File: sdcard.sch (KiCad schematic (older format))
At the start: 8 parts, among them J10 Micro_SD_Card

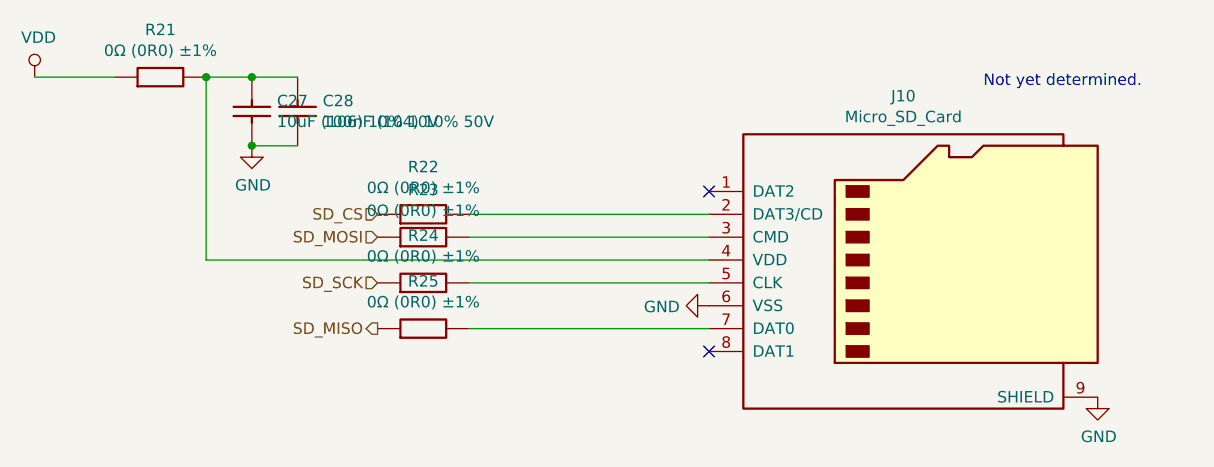
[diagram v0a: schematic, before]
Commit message: 20191114
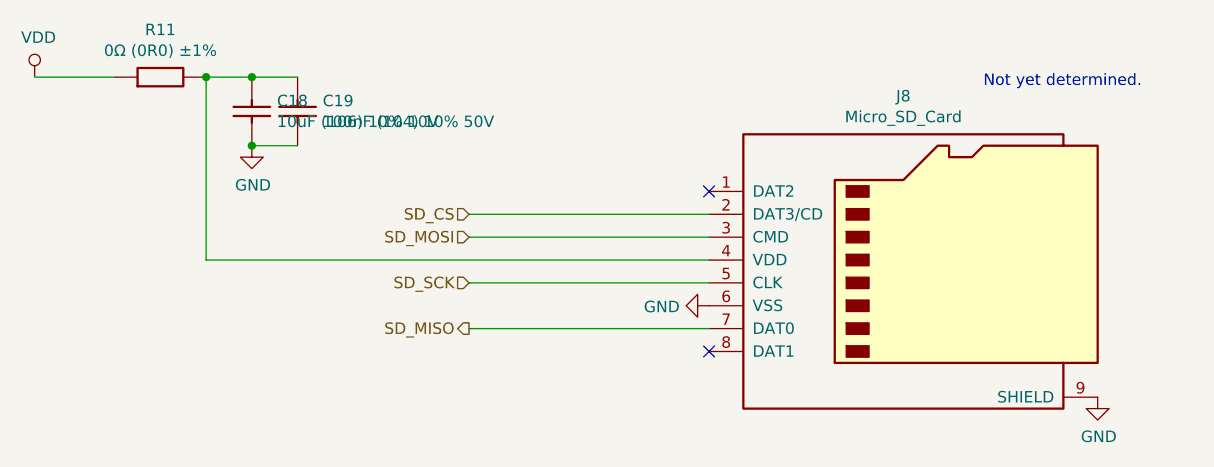
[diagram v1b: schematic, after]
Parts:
- removed R22, R23, R24, R25: 0603_0Ω__0R0_1%, lc_lib:0603_R, symbol lc_RES:0603_0Ω__0R0_1%
- J8: renamed from J10; footprint (none) -> Connector_Card:microSD_HC_Hirose_DM3D-SF
- renumbered C27 to C18, C28 to C19, R21 to R11
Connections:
- net SD_CS: now also J8.2 (DAT3/CD)
- net SD_MISO: now also J8.7 (DAT0)
- net SD_MOSI: now also J8.3 (CMD)
- net SD_SCK: now also J8.5 (CLK)
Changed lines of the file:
@@
 $Descr A4 11693 8268
 encoding utf-8
-Sheet 5 9
+Sheet 4 9
 Title ""
 Date ""
@@
 Comment4 ""
 $EndDescr
-Text HLabel 3550 3700 0    50   Output ~ 0
+Text HLabel 3950 3700 0    50   Output ~ 0
 SD_MISO
-Text HLabel 3550 3200 0    50   Input ~ 0
+Text HLabel 3950 3200 0    50   Input ~ 0
 SD_CS
-Text HLabel 3550 3300 0    50   Input ~ 0
+Text HLabel 3950 3300 0    50   Input ~ 0
 SD_MOSI
-Text HLabel 3550 3500 0    50   Input ~ 0
+Text HLabel 3950 3500 0    50   Input ~ 0
 SD_SCK
 $Comp
@@
 P 6700 4000
 AR Path="/5DF49590/5DCF2E63" Ref="#PWR?"  Part="1"
-AR Path="/5DCEE376/5DCF2E63" Ref="#PWR058"  Part="1"
-F 0 "#PWR058" H 6700 3750 50  0001 C CNN
+AR Path="/5DCEE376/5DCF2E63" Ref="#PWR038"  Part="1"
+F 0 "#PWR038" H 6700 3750 50  0001 C CNN
 F 1 "GND" H 6705 3827 50  0000 C CNN
 F 2 "" H 6700 4000 50  0001 C CNN
@@
 P 2600 2600
 AR Path="/5DF49590/5DCF2E76" Ref="R?"  Part="1"
-AR Path="/5DCEE376/5DCF2E76" Ref="R21"  Part="1"
-F 0 "R21" H 2600 2807 50  0000 C CNN
+AR Path="/5DCEE376/5DCF2E76" Ref="R11"  Part="1"
+F 0 "R11" H 2600 2807 50  0000 C CNN
 F 1 "0603_0Ω__0R0_1%" H 2450 2790 50  0001 L BNN
 F 2 "lc_lib:0603_R" H 2400 2360 50  0001 L BNN
@@
 P 5000 3600
 AR Path="/5DF49590/5DCF2EF5" Ref="#PWR?"  Part="1"
-AR Path="/5DCEE376/5DCF2EF5" Ref="#PWR057"  Part="1"
-F 0 "#PWR057" H 5000 3350 50  0001 C CNN
+AR Path="/5DCEE376/5DCF2EF5" Ref="#PWR037"  Part="1"
+F 0 "#PWR037" H 5000 3350 50  0001 C CNN
 F 1 "GND" V 5005 3472 50  0000 R CNN
 F 2 "" H 5000 3600 50  0001 C CNN
@@
 P 3000 2400
 AR Path="/5DF49590/5DCF2F02" Ref="C?"  Part="1"
-AR Path="/5DCEE376/5DCF2F02" Ref="C27"  Part="1"
-F 0 "C27" V 3304 2510 50  0000 L CNN
+AR Path="/5DCEE376/5DCF2F02" Ref="C18"  Part="1"
+F 0 "C18" V 3304 2510 50  0000 L CNN
 F 1 "0603_10uF__106_10%_10V" H 3049 2630 50  0001 L BNN
 F 2 "lc_lib:0603_C" H 2999 2120 50  0001 L BNN
@@
 P 3200 2400
 AR Path="/5DF49590/5DCF2F11" Ref="C?"  Part="1"
-AR Path="/5DCEE376/5DCF2F11" Ref="C28"  Part="1"
-F 0 "C28" V 3504 2510 50  0000 L CNN
+AR Path="/5DCEE376/5DCF2F11" Ref="C19"  Part="1"
+F 0 "C19" V 3504 2510 50  0000 L CNN
 F 1 "0603_100nF__104_10%_50V" H 3249 2630 50  0001 L BNN
 F 2 "lc_lib:0603_C" H 3199 2120 50  0001 L BNN
@@
 P 3000 2900
 AR Path="/5DF49590/5DCF2F1A" Ref="#PWR?"  Part="1"
-AR Path="/5DCEE376/5DCF2F1A" Ref="#PWR056"  Part="1"
-F 0 "#PWR056" H 3000 2650 50  0001 C CNN
+AR Path="/5DCEE376/5DCF2F1A" Ref="#PWR036"  Part="1"
+F 0 "#PWR036" H 3000 2650 50  0001 C CNN
 F 1 "GND" H 3005 2727 50  0000 C CNN
 F 2 "" H 3000 2900 50  0001 C CNN
@@
 Text Notes 6200 2650 0    50   ~ 0
 Not yet determined.
-$Comp
-L lc_RES:0603_0Ω__0R0_1% R?
-U 1 1 5DCF2F3A
-P 3750 3200
-AR Path="/5DF49590/5DCF2F3A" Ref="R?"  Part="1"
-AR Path="/5DCEE376/5DCF2F3A" Ref="R22"  Part="1"
-F 0 "R22" H 3750 3407 50  0000 C CNN
-F 1 "0603_0Ω__0R0_1%" H 3600 3390 50  0001 L BNN
-F 2 "lc_lib:0603_R" H 3550 2960 50  0001 L BNN
-F 3 "http://www.szlcsc.com/product/details_21903.html" H 3550 3060 50  0001 L BNN
-F 4 "贴片电阻" H 3750 3200 50  0001 C CNN "description"
-F 5 "供应商链接" H 3550 2860 50  0001 L BNN "ComponentLink1Description"
-F 6 "0603" H 3550 2760 50  0001 L BNN "Package"
-F 7 "LC" H 3550 2660 50  0001 L BNN "Supplier"
-F 8 "C21189" H 3550 2560 50  0001 L BNN "SuppliersPartNumber"
-F 9 "" H 3550 2460 50  0001 L BNN "Notepad"
-F 10 "0Ω (0R0) ±1%" H 3750 3316 50  0000 C CNN "Comment"
-	1    3750 3200
-	1    0    0    -1
-$EndComp
-$Comp
-L lc_RES:0603_0Ω__0R0_1% R?
-U 1 1 5DCF2F47
-P 3750 3300
-AR Path="/5DF49590/5DCF2F47" Ref="R?"  Part="1"
-AR Path="/5DCEE376/5DCF2F47" Ref="R23"  Part="1"
-F 0 "R23" H 3750 3507 50  0000 C CNN
-F 1 "0603_0Ω__0R0_1%" H 3600 3490 50  0001 L BNN
-F 2 "lc_lib:0603_R" H 3550 3060 50  0001 L BNN
-F 3 "http://www.szlcsc.com/product/details_21903.html" H 3550 3160 50  0001 L BNN
-F 4 "贴片电阻" H 3750 3300 50  0001 C CNN "description"
-F 5 "供应商链接" H 3550 2960 50  0001 L BNN "ComponentLink1Description"
-F 6 "0603" H 3550 2860 50  0001 L BNN "Package"
-F 7 "LC" H 3550 2760 50  0001 L BNN "Supplier"
-F 8 "C21189" H 3550 2660 50  0001 L BNN "SuppliersPartNumber"
-F 9 "" H 3550 2560 50  0001 L BNN "Notepad"
-F 10 "0Ω (0R0) ±1%" H 3750 3416 50  0000 C CNN "Comment"
-	1    3750 3300
-	1    0    0    -1
-$EndComp
-$Comp
-L lc_RES:0603_0Ω__0R0_1% R?
-U 1 1 5DCF2F54
-P 3750 3500
-AR Path="/5DF49590/5DCF2F54" Ref="R?"  Part="1"
-AR Path="/5DCEE376/5DCF2F54" Ref="R24"  Part="1"
-F 0 "R24" H 3750 3707 50  0000 C CNN
-F 1 "0603_0Ω__0R0_1%" H 3600 3690 50  0001 L BNN
-F 2 "lc_lib:0603_R" H 3550 3260 50  0001 L BNN
-F 3 "http://www.szlcsc.com/product/details_21903.html" H 3550 3360 50  0001 L BNN
-F 4 "贴片电阻" H 3750 3500 50  0001 C CNN "description"
-F 5 "供应商链接" H 3550 3160 50  0001 L BNN "ComponentLink1Description"
-F 6 "0603" H 3550 3060 50  0001 L BNN "Package"
-F 7 "LC" H 3550 2960 50  0001 L BNN "Supplier"
-F 8 "C21189" H 3550 2860 50  0001 L BNN "SuppliersPartNumber"
-F 9 "" H 3550 2760 50  0001 L BNN "Notepad"
-F 10 "0Ω (0R0) ±1%" H 3750 3616 50  0000 C CNN "Comment"
-	1    3750 3500
-	1    0    0    -1
-$EndComp
-$Comp
-L lc_RES:0603_0Ω__0R0_1% R?
-U 1 1 5DCF2F61
-P 3750 3700
-AR Path="/5DF49590/5DCF2F61" Ref="R?"  Part="1"
-AR Path="/5DCEE376/5DCF2F61" Ref="R25"  Part="1"
-F 0 "R25" H 3750 3907 50  0000 C CNN
-F 1 "0603_0Ω__0R0_1%" H 3600 3890 50  0001 L BNN
-F 2 "lc_lib:0603_R" H 3550 3460 50  0001 L BNN
-F 3 "http://www.szlcsc.com/product/details_21903.html" H 3550 3560 50  0001 L BNN
-F 4 "贴片电阻" H 3750 3700 50  0001 C CNN "description"
-F 5 "供应商链接" H 3550 3360 50  0001 L BNN "ComponentLink1Description"
-F 6 "0603" H 3550 3260 50  0001 L BNN "Package"
-F 7 "LC" H 3550 3160 50  0001 L BNN "Supplier"
-F 8 "C21189" H 3550 3060 50  0001 L BNN "SuppliersPartNumber"
-F 9 "" H 3550 2960 50  0001 L BNN "Notepad"
-F 10 "0Ω (0R0) ±1%" H 3750 3816 50  0000 C CNN "Comment"
-	1    3750 3700
-	1    0    0    -1
-$EndComp
 Connection ~ 2800 2600
 Wire Wire Line
 	2800 3400 5000 3400
 $Comp
-L power:VDD #PWR055
+L power:VDD #PWR035
 U 1 1 5DCF4828
 P 2050 2600
-F 0 "#PWR055" H 2050 2450 50  0001 C CNN
+F 0 "#PWR035" H 2050 2450 50  0001 C CNN
 F 1 "VDD" H 2067 2773 50  0000 C CNN
 F 2 "" H 2050 2600 50  0001 C CNN
@@
 	2050 2600 2400 2600
 $Comp
-L Connector:Micro_SD_Card J10
+L Connector:Micro_SD_Card J8
 U 1 1 5DD26AA4
 P 5900 3400
-F 0 "J10" H 5850 4117 50  0000 C CNN
+F 0 "J8" H 5850 4117 50  0000 C CNN
 F 1 "Micro_SD_Card" H 5850 4026 50  0000 C CNN
-F 2 "" H 7050 3700 50  0001 C CNN
+F 2 "Connector_Card:microSD_HC_Hirose_DM3D-SF" H 7050 3700 50  0001 C CNN
 F 3 "http://katalog.we-online.de/em/datasheet/693072010801.pdf" H 5900 3400 50  0001 C CNN
 	1    5900 3400
